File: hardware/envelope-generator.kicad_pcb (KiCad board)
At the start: 2 copper layers, 127 x 76.2 mm, 87 parts, among them J1 Power bus, J10 EG 1 Out, J2 SWD, J3 Serial Dongle, J4 EG 2 Out, J5 Gate 1 In, J6 CAN, J7 Gate 2 In, SW1 Gate Src, SW2 EG Modes, SW3 NRST, U1 TL072, U2 MC34063AD, U3 TL072, U4 LM4040DBZ-3, U8 STM32C092KCT6, U9 TCAN3413, Y1 48 MHz

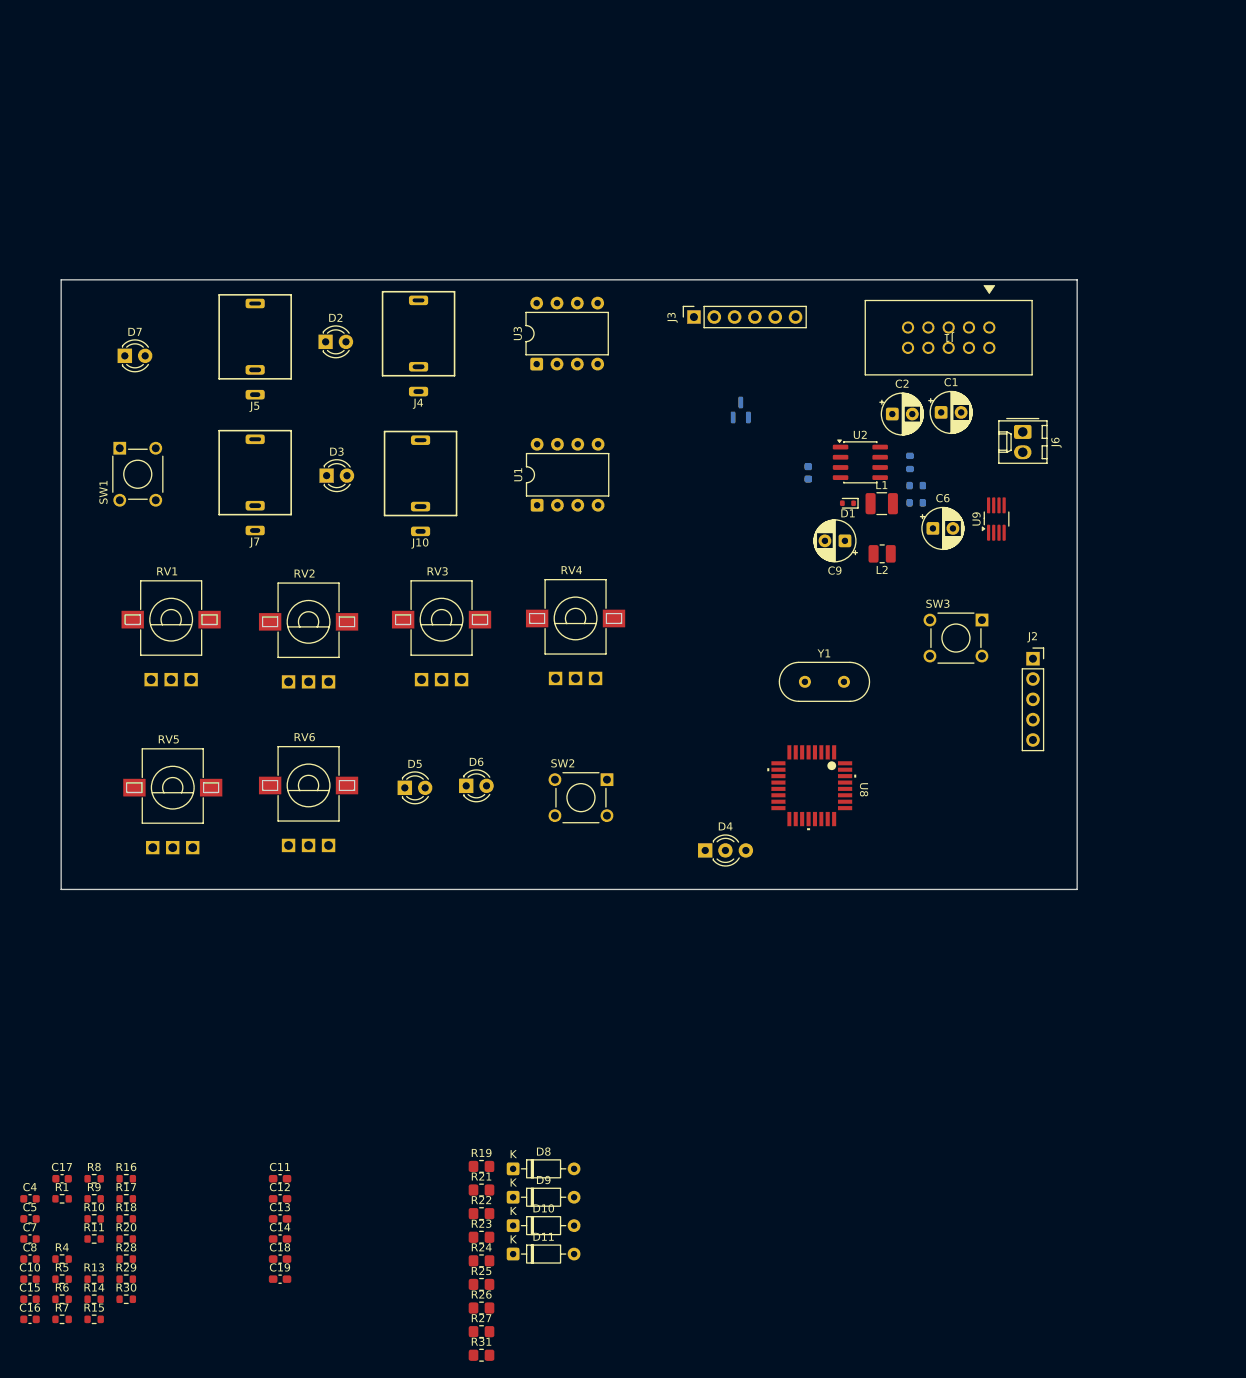
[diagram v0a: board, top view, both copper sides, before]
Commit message: PCB design the first iteration
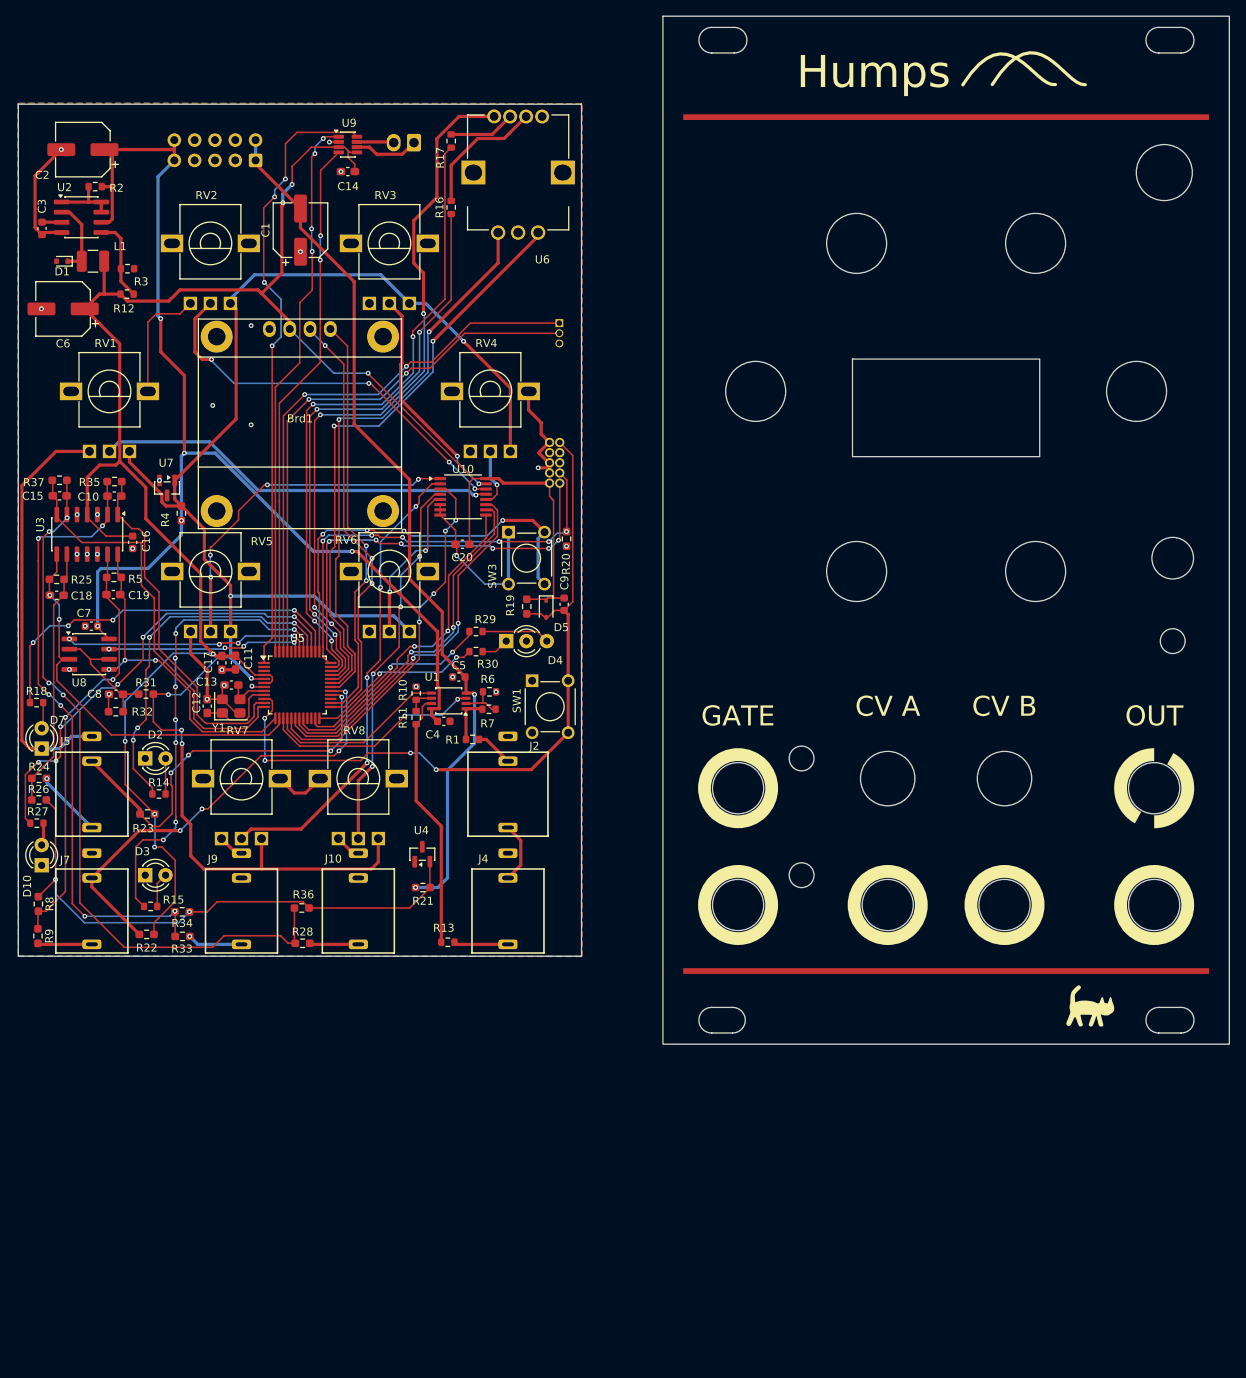
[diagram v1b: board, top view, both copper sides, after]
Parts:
- removed D11, D8, D9: 1N4148W, Diode_THT:D_DO-35_SOD27_P7.62mm_Horizontal
- removed D6: Mode 1, LED_THT:LED_D3.0mm
- removed L2: 150u, Inductor_SMD:L_1008_2520Metric
- removed SW2: EG Modes, Tactile_Switches:SW4_1825910-B_TEC
- added Brd1: SSD1306, SSD1306:128x64OLED_aki, F.Cu at (99.7, 76.6)
- added C20: 100n, Capacitor_SMD:C_0603_1608Metric_Pad1.08x0.95mm_HandSolder, F.Cu at (120.0, 93.6)
- added J8: SWD, Connector_Synth:CONN_2x10_3220-10-0100-00_CNC, B.Cu at (130.9, 86.0)
- added J9: CV 1 In, Synth:Thonkiconn, F.Cu at (92.4, 138.7)
- added R32: 15k, Resistor_SMD:R_0603_1608Metric_Pad0.98x0.95mm_HandSolder, F.Cu at (76.7, 114.6)
- added R33: 100k, Resistor_SMD:R_0603_1608Metric_Pad0.98x0.95mm_HandSolder, F.Cu at (85.0, 142.7)
- added R34: 36k, Resistor_SMD:R_0603_1608Metric_Pad0.98x0.95mm_HandSolder, F.Cu at (85.0, 139.6)
- added R35: 18k, Resistor_SMD:R_0603_1608Metric_Pad0.98x0.95mm_HandSolder, F.Cu at (76.5, 85.8)
- added R36: 36k, Resistor_SMD:R_0603_1608Metric_Pad0.98x0.95mm_HandSolder, F.Cu at (99.9, 139.1)
- added R37: 18k, Resistor_SMD:R_0603_1608Metric_Pad0.98x0.95mm_HandSolder, F.Cu at (69.6, 85.7)
- added REF**: 3.5mm dual channel, Panel_Utilities:3.5mm dual thick, F.Cu at (206.5, 124.1)
- added REF**: knob 14mm alpha, Panel_Utilities:knob 14mm alpha, F.Cu at (204.3, 74.5)
- added REF**: knob shaft, Panel_Utilities:knob shaft, F.Cu at (187.8, 122.9)
- added REF**: knob 14mm alpha, Panel_Utilities:knob 14mm alpha, F.Cu at (156.7, 74.5)
- added REF**: logo-6mm, GajeLogo:logo-6mm, F.Cu at (198.0, 151.7)
- added REF**: 3.5mm single channel, Panel_Utilities:3.5mm single thick, F.Cu at (173.2, 138.7)
- added REF**: knob 14mm alpha, Panel_Utilities:knob 14mm alpha, F.Cu at (169.3, 56.0)
- added REF**: knob 14mm alpha, Panel_Utilities:knob 14mm alpha, F.Cu at (191.7, 56.0)
- added REF**: 3.5mm single channel, Panel_Utilities:3.5mm single thick, F.Cu at (187.8, 138.7)
- added REF**: LED 3mm, Panel_Utilities:LED 3mm, F.Cu at (208.8, 105.8)
- added REF**: SW Push Button, Panel_Utilities:SW Push Button, F.Cu at (208.8, 95.4)
- added REF**: LED 3mm, Panel_Utilities:LED 3mm, F.Cu at (162.4, 135.0)
- added REF**: 3.5mm single channel, Panel_Utilities:3.5mm single thick, F.Cu at (154.5, 124.1)
- added REF**: 3.5mm single channel, Panel_Utilities:3.5mm single thick, F.Cu at (206.5, 138.7)
- added REF**: logo-4mm, GajeLogo:logo-4mm, B.Cu at (72.4, 48.3)
- added REF**: 3.5mm single channel, Panel_Utilities:3.5mm single thick, F.Cu at (154.5, 138.7)
- added REF**: knob 14mm alpha, Panel_Utilities:knob 14mm alpha, F.Cu at (169.3, 97.1)
- added REF**: PEL12D, Panel_Utilities:PEL12D, F.Cu at (207.7, 47.2)
- added REF**: knob 14mm alpha, Panel_Utilities:knob 14mm alpha, F.Cu at (191.7, 97.1)
- added REF**: knob shaft, Panel_Utilities:knob shaft, F.Cu at (173.2, 122.9)
- added REF**: HP14, EuroRackPanels:HP14, F.Cu at (145.1, 27.6)
- added REF**: LED 3mm, Panel_Utilities:LED 3mm, F.Cu at (162.4, 120.4)
- added RV7: 10k, Synth:ALPHA_9MM, F.Cu at (92.4, 122.9)
- added RV8: 10k, Synth:ALPHA_9MM, F.Cu at (107.0, 122.9)
- added SSD1306: 128x64OLED, Panel_Utilities:128x64 OLED Window, F.Cu at (180.5, 76.6)
- added U10: CD4051B, Package_SO:TSSOP-16_4.4x5mm_P0.65mm, F.Cu at (120.1, 87.7)
- added U5: STM32G0B1CBTx, Package_QFP:LQFP-48_7x7mm_P0.5mm, F.Cu at (99.4, 111.2)
- added U6: PEL12D-4225S-S2024, PEL12D:TO_4225S-S2024, F.Cu at (127.0, 47.2)
- added U7: LM4040DBZ-3, Package_TO_SOT_SMD:SOT-23, F.Cu at (83.1, 86.6)
- C1, C2, C6: footprint Capacitor_THT:CP_Radial_D5.0mm_P2.50mm -> Capacitor_SMD:CP_Elec_6.3x5.4_Nichicon
- C10, C15: value 1n -> 4.7n; footprint Capacitor_SMD:C_0603_1608Metric -> Capacitor_SMD:C_0603_1608Metric_Pad1.08x0.95mm_HandSolder
- C17: value 100n -> 2.2u; footprint Capacitor_SMD:C_0603_1608Metric -> Capacitor_SMD:C_0603_1608Metric_Pad1.08x0.95mm_HandSolder
- C18, C19: value 2.2n -> 1n
- C3, R12, R2, R3: moved to F.Cu
- C7: value 1n -> 100n
- C8: value 1n -> 1u; footprint Capacitor_SMD:C_0603_1608Metric -> Capacitor_SMD:C_0603_1608Metric_Pad1.08x0.95mm_HandSolder
- C9: value 47u -> 10u; footprint Capacitor_THT:CP_Radial_D5.0mm_P2.50mm -> Capacitor_SMD:C_0603_1608Metric
- D10: value 1N4148W -> Analog SRC 2; footprint Diode_THT:D_DO-35_SOD27_P7.62mm_Horizontal -> Synth:LED_D3.0mm
- D2, D3: footprint LED_THT:LED_D3.0mm -> Synth:LED_D3.0mm
- D5: value Mode 0 -> 1N4148WS; footprint LED_THT:LED_D3.0mm -> Diode_SMD:D_SOD-323
- D7: value Analog Ind -> Analog SRC 1; footprint LED_THT:LED_D3.0mm -> Synth:LED_D3.0mm
- J1: footprint Synth:CONN10_302-S101_OST -> Connector_IDC:IDC-Header_2x05_P2.54mm_Vertical; moved to B.Cu
- J10: value EG 1 Out -> CV 2 In
- J2: value SWD -> Dual or Voice 1 Out; footprint Connector_PinSocket_2.54mm:PinSocket_1x05_P2.54mm_Vertical -> Synth:Thonkiconn_Stereo
- J3: value Serial Dongle -> Conn_01x03_Socket; footprint Connector_PinSocket_2.54mm:PinSocket_1x06_P2.54mm_Vertical -> Connector_PinSocket_1.27mm:PinSocket_1x03_P1.27mm_Vertical; moved to B.Cu
- J6: moved to B.Cu
- R10, R6: value 20k -> 10k
- R16, R17: value 180 -> 680
- R19, R21, R24, R26: footprint Resistor_SMD:R_0805_2012Metric_Pad1.20x1.40mm_HandSolder -> Resistor_SMD:R_0603_1608Metric_Pad0.98x0.95mm_HandSolder
- R20: footprint Resistor_SMD:R_0603_1608Metric -> Resistor_SMD:R_0603_1608Metric_Pad0.98x0.95mm_HandSolder
- R22: value 100k -> 470k; footprint Resistor_SMD:R_0805_2012Metric_Pad1.20x1.40mm_HandSolder -> Resistor_SMD:R_0603_1608Metric_Pad0.98x0.95mm_HandSolder
- R23: value 36k -> 470k; footprint Resistor_SMD:R_0805_2012Metric_Pad1.20x1.40mm_HandSolder -> Resistor_SMD:R_0603_1608Metric_Pad0.98x0.95mm_HandSolder
- R25: value 39k -> 36k; footprint Resistor_SMD:R_0805_2012Metric_Pad1.20x1.40mm_HandSolder -> Resistor_SMD:R_0603_1608Metric_Pad0.98x0.95mm_HandSolder
- R27: value 39k -> 180; footprint Resistor_SMD:R_0805_2012Metric_Pad1.20x1.40mm_HandSolder -> Resistor_SMD:R_0603_1608Metric
- R28: value 10k -> 100k; footprint Resistor_SMD:R_0603_1608Metric -> Resistor_SMD:R_0603_1608Metric_Pad0.98x0.95mm_HandSolder
- R31: value 1Meg -> 3.3k; footprint Resistor_SMD:R_0805_2012Metric_Pad1.20x1.40mm_HandSolder -> Resistor_SMD:R_0603_1608Metric_Pad0.98x0.95mm_HandSolder
- R4: value 20k -> 10k; footprint Resistor_SMD:R_0603_1608Metric -> Resistor_SMD:R_0603_1608Metric_Pad0.98x0.95mm_HandSolder
- R5, R8: value 20k -> 36k; footprint Resistor_SMD:R_0603_1608Metric -> Resistor_SMD:R_0603_1608Metric_Pad0.98x0.95mm_HandSolder
- R9: value 20k -> 100k; footprint Resistor_SMD:R_0603_1608Metric -> Resistor_SMD:R_0603_1608Metric_Pad0.98x0.95mm_HandSolder
- SW1: value Gate Src -> USER_SW
- SW3: value NRST -> USER_SW
- U1: footprint Package_DIP:DIP-8_W7.62mm -> Package_SO:TSSOP-8_3x3mm_P0.65mm
- U3: value TL072 -> MCP6004; footprint Package_DIP:DIP-8_W7.62mm -> Package_SO:SOIC-14_3.9x8.7mm_P1.27mm
- U4: value LM4040DBZ-3 -> LM4040DBZ-10; moved to F.Cu
- U8: value STM32C092KCT6 -> LM393; footprint stm32c092kct6:LQFP-32_STM-M -> Package_SO:SOIC-8_3.9x4.9mm_P1.27mm
- U9: footprint Package_TO_SOT_SMD:TSOT-23-8_HandSoldering -> Package_TO_SOT_SMD:TSOT-23-8
- Y1: value 48 MHz -> 16MHz; footprint Crystal:Crystal_HC49-4H_Vertical -> Crystal:Crystal_SMD_Abracon_ABM8G-4Pin_3.2x2.5mm
- moved R17 138.3 mm to (118.6, 43.2), turned to -90 degrees
- moved C14 133.7 mm to (105.7, 47.1), turned to 180 degrees
- moved R16 128.0 mm to (118.6, 51.5), turned to 90 degrees
- moved C6 112.1 mm to (70.1, 64.2), turned to 180 degrees
- moved R2 107.5 mm to (74.1, 49.0), turned to 180 degrees
- moved C2 106.4 mm to (72.6, 44.3), turned to 180 degrees
- moved R20 103.4 mm to (133.0, 93.0), turned to 90 degrees
- moved L1 103.2 mm to (73.8, 58.3)
- moved R25 102.9 mm to (69.3, 98.0)
- moved D1 102.8 mm to (70.0, 58.3)
- moved R3 102.2 mm to (78.1, 59.2)
- moved U2 102.1 mm to (72.4, 52.8)
- moved R12 102.0 mm to (78.1, 62.4), turned to 0 degrees
- moved C3 100.5 mm to (67.5, 54.2)
- moved C15 100.5 mm to (69.7, 87.6), turned to 180 degrees
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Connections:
- C10 pad 1: Net-(C10-Pad1) -> Net-(U3A--)
- C10 pad 2: GND -> /ADC_CV_1
- C12 pad 2: Net-(U8-PC15-OSCX_OUT) -> /OSC_OUT
- C13 pad 2: Net-(U8-PC14-OSCX_IN) -> /OSC_IN
- C15 pad 1: Net-(U1B-+) -> Net-(U3B--)
- C15 pad 2: GND -> /ADC_CV_2
- C16 pad 1: +12V -> +3.3V
- C17 pad 1: GND -> +3.3V
- C17 pad 2: -12V -> GND
- C18 pad 1: Net-(U3A--) -> Net-(U3C--)
- C18 pad 2: Net-(C18-Pad2) -> /ADC_GATE_1
- C19 pad 1: Net-(U3B--) -> Net-(U3D--)
- C19 pad 2: Net-(C19-Pad2) -> /ADC_GATE_2
- C7 pad 1: Net-(C7-Pad1) -> +12V
- C8 pad 1: Net-(U1A-+) -> /GATE_REF
- C9 pad 1: +3.3VA -> +3.3V
- C9 pad 2: GND -> /NRST
- D10 pad 1: +3.3VA -> GND
- D10 pad 2: /ADC_GATE_2 -> Net-(D10-A)
- D5 pad 1: GND -> +3.3V
- D5 pad 2: Net-(D5-A) -> /NRST
- J10 pad T: /EG_1_OUT -> Net-(J10-PadT)
- J3 pad 1: unconnected-(J3-Pin_1-Pad1) -> /UART_RX
- J3 pad 2: /UART_RX -> /UART_TX
- J3 pad 3: /UART_TX -> GND
- J4 pad TN: unconnected-(J4-PadTN) -> Net-(J2-PadT)
- J5 pad TN: unconnected-(J5-PadTN) -> /GATE_SRC_SW_1
- J7 pad TN: /SW_GATE_2 -> /GATE_SRC_SW_2
- R16 pad 1: /IND_EG_MODE_0 -> /ENCODER_IND_GREEN
- R16 pad 2: Net-(D5-A) -> Net-(R16-Pad2)
- R17 pad 1: /IND_EG_MODE_1 -> Net-(R17-Pad1)
- R17 pad 2: Net-(D6-A) -> /ENCODER_IND_RED
- R18 pad 1: /IND_ANALOG_GATE -> /IND_ANALOG_GATE_1
- R20 pad 1: /ADC_GATE_1 -> GND
- R20 pad 2: Net-(C18-Pad2) -> /SWCLK
- R22 pad 1: Net-(U3B--) -> /GATE_SRC_SW_2
- R22 pad 2: Net-(J7-PadT) -> +3.3V
- R23 pad 1: /AREF_-3V -> /GATE_SRC_SW_1
- R23 pad 2: Net-(U3B--) -> +3.3V
- R24 pad 1: Net-(U3A--) -> Net-(U3C--)
- R25 pad 1: Net-(C18-Pad2) -> /ADC_GATE_1
- R25 pad 2: Net-(U3A--) -> Net-(U3C--)
- R26 pad 2: Net-(U3A--) -> Net-(U3C--)
- R27 pad 1: Net-(C19-Pad2) -> /IND_ANALOG_GATE_2
- R27 pad 2: Net-(U3B--) -> Net-(D10-A)
- R28 pad 1: /ADC_GATE_2 -> Net-(U3B--)
- R28 pad 2: Net-(C19-Pad2) -> Net-(J10-PadT)
- R31 pad 1: +3.3VA -> /GATE_REF
- R31 pad 2: /SW_GATE_2 -> /AREF_3V
- R4 pad 1: Net-(C7-Pad1) -> /AREF_3V
- R4 pad 2: /TIM3_CH1 -> +12V
- R5 pad 1: Net-(U1A-+) -> /ADC_GATE_2
- R5 pad 2: Net-(C7-Pad1) -> Net-(U3D--)
- R8 pad 1: Net-(C10-Pad1) -> /AREF_-3V
- R8 pad 2: /TIM3_CH4 -> Net-(U3D--)
- R9 pad 1: Net-(U1B-+) -> Net-(U3D--)
- R9 pad 2: Net-(C10-Pad1) -> Net-(J7-PadT)
- RV1 pad 2: /ADC_A -> /A
- RV1 pad 3: +3.3VA -> /AREF_3V
- RV2 pad 2: /ADC_D -> /D
- RV2 pad 3: +3.3VA -> /AREF_3V
- RV3 pad 2: /ADC_S -> /S
- RV3 pad 3: +3.3VA -> /AREF_3V
- RV4 pad 2: /ADC_R -> /R
- RV4 pad 3: +3.3VA -> /AREF_3V
- RV5 pad 2: /ADC_D0 -> /D0
- RV5 pad 3: +3.3VA -> /AREF_3V
- RV6 pad 2: /ADC_S0 -> /S0
- RV6 pad 3: +3.3VA -> /AREF_3V
- SW1 pad 3: /SW_GATE_SRC -> /NRST
- SW1 pad 4: /SW_GATE_SRC -> /NRST
- SW3 pad 3: /NRST -> /USER_SW
- SW3 pad 4: /NRST -> /USER_SW
- U1 pad 3: Net-(U1A-+) -> /DAC_OUT_1
- U1 pad 5: Net-(U1B-+) -> /DAC_OUT_2
- U3 pad 1: Net-(C18-Pad2) -> /ADC_CV_1
- U3 pad 4: -12V -> +3.3V
- U3 pad 7: Net-(C19-Pad2) -> /ADC_CV_2
- U3 pad 8: +12V -> /ADC_GATE_1
- U8 pad 1: /SW_GATE_2 -> /GATE_TRIGGER_1
- U8 pad 2: Net-(U8-PC14-OSCX_IN) -> /GATE_REF
- U8 pad 3: Net-(U8-PC15-OSCX_OUT) -> /ADC_GATE_1
- U8 pad 4: +3.3V -> GND
- U8 pad 5: GND -> /ADC_GATE_2
- U8 pad 6: /NRST -> /GATE_REF
- U8 pad 7: /ADC_A -> /GATE_TRIGGER_2
- U8 pad 8: /ADC_D -> +12V
- Y1 pad 1: Net-(U8-PC15-OSCX_OUT) -> /OSC_OUT
- Y1 pad 2: Net-(U8-PC14-OSCX_IN) -> GND
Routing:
- net +3.3V: track 0.00 -> 256.6 mm, vias 0 -> 7
- net /AREF_3V: track 0.00 -> 208.7 mm, vias 0 -> 6
- net GND: track 0.00 -> 153.4 mm, vias 0 -> 28
- net +12V: track 0.00 -> 147.3 mm, vias 0 -> 5
- net -12V: track 0.00 -> 110.0 mm, vias 0 -> 2
- net /NRST: track 0.00 -> 93.0 mm, vias 0 -> 4
- net Net-(U3B--): track 0.00 -> 91.2 mm, vias 0 -> 4
- net /ENCODER_SW: track 0.00 -> 91.0 mm, vias 0 -> 4
- net /ENCODER_IND_RED: track 0.00 -> 81.0 mm, vias 0 -> 4
- net Net-(U3A--): track 0.00 -> 78.8 mm, vias 0 -> 6
- net /CAN_STB: track 0.00 -> 77.7 mm, vias 0 -> 4
- net /ENCODER_B: track 0.00 -> 73.3 mm, vias 0 -> 2
- net /ENCODER_IND_GREEN: track 0.00 -> 72.8 mm, vias 0 -> 4
- net /ENCODER_A: track 0.00 -> 71.2 mm, vias 0 -> 2
- net /AREF_-3V: track 0.00 -> 69.3 mm, vias 0 -> 2
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- added copper zone on B.Cu, net GND
- added copper zone on F.Cu, net GND
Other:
- board size 127 x 76.2 mm -> 70.8 x 128.5 mm
- board text added: "<RX"
- board text added: ">TX"
- board text added: "Analog3 Humps-D Rev. 1"
- board text added: "CV A"
- board text added: "CV B"
- board text added: "GATE"
- board text added: "GND"
- board text added: "Humps"
- board text added: "OUT"
- board text added: "SWD"
- board text added: "Serial"
